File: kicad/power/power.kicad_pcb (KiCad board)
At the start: 2 copper layers, 115.3 x 75.4 mm, 31 parts, among them J1 Conn_01x06, J10 Conn_01x06, J11 Conn_01x06, J12 Conn_01x06, J13 Conn_01x06, J2 AudioJack3, J3 USB_C_Receptacle, J4 AudioJack3, J5 AudioJack3, J6 Conn_01x05_Male, J7 Screw_Terminal_01x02, J9 Conn_01x04_Male, U1 LM4565F-GE2, U2 LM4565F-GE2, U3 LM4565F-GE2, U4 LM4565F-GE2, U5 LF353DR

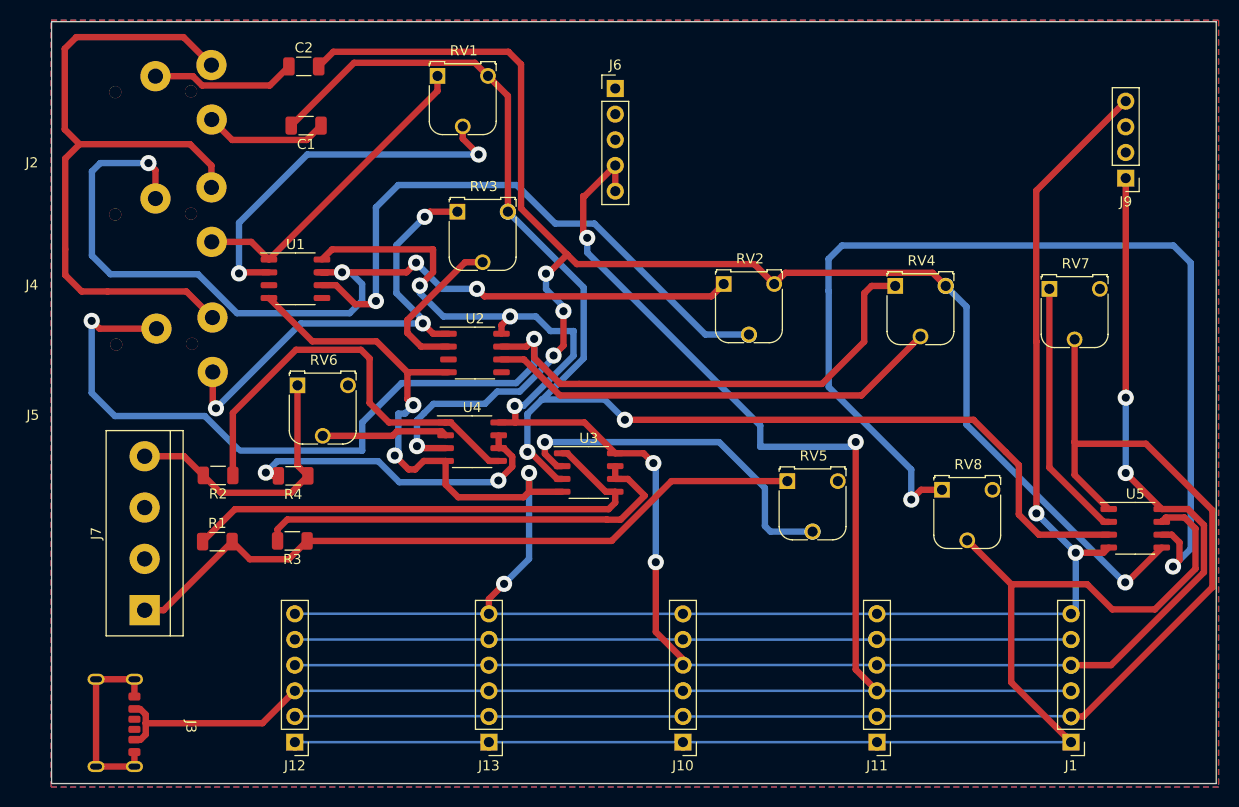
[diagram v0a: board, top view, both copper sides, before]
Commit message: Power PCB revisions
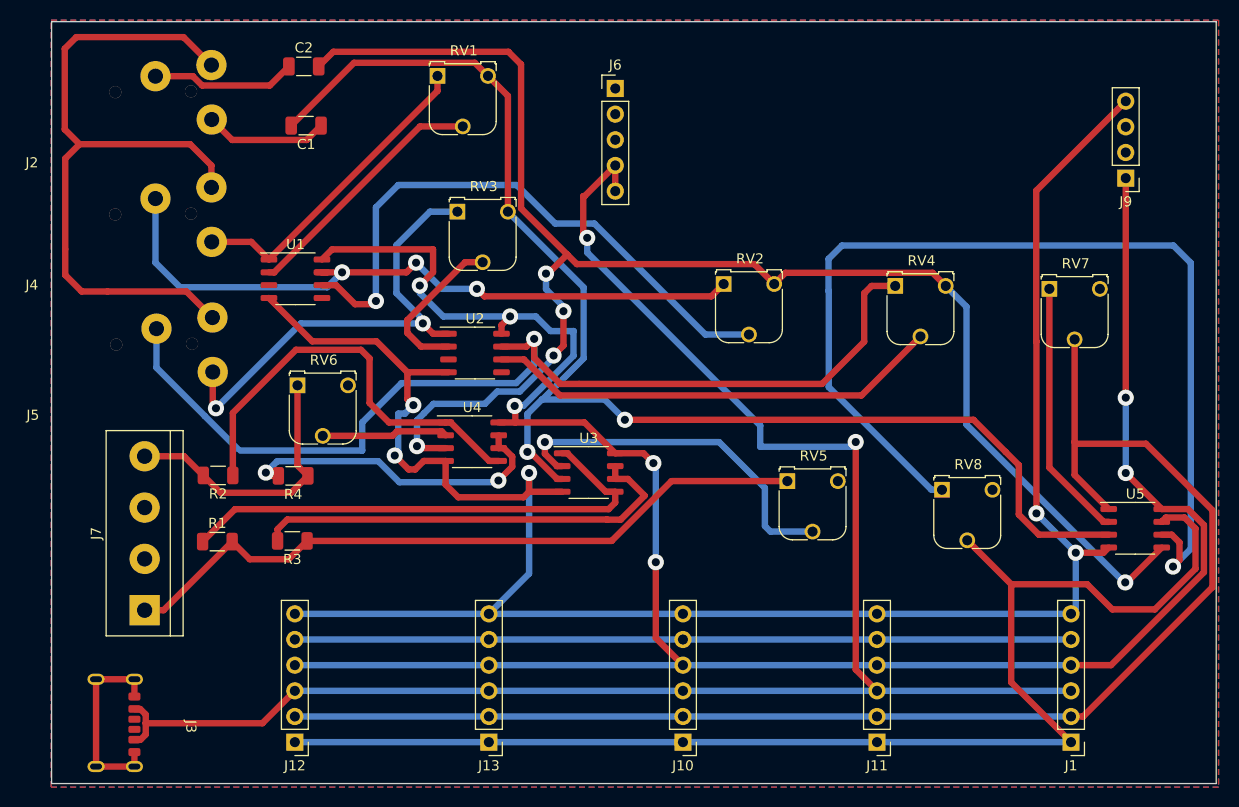
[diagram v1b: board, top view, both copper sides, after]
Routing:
- net audio_right: track 130.0 -> 206.8 mm, vias 4 -> 0
- net +5V: track 171.8 -> 248.6 mm, vias 7 -> 2
- net +15V: track 222.8 -> 299.6 mm, vias 12 -> 7
- net GND: track 168.3 -> 245.1 mm, vias 5 -> 0
- net audio_lefT: track 138.4 -> 215.0 mm, vias 5 -> 0
- net -15V: track 204.5 -> 280.6 mm, vias 11 -> 5
- net Net-(J4-PadR): track 94.9 -> 69.5 mm, vias 4 -> 3
- net Net-(J5-PadR): track 116.5 -> 101.1 mm, vias 2 -> 1
- net Net-(RV1-Pad2): track 38.0 -> 25.2 mm, vias 2 -> 0
- net Net-(RV8-Pad1): track 103.3 -> 100.7 mm, vias 2 -> 1
- net audio_in_R: vias 6 -> 5
- net audio_in_L: vias 3 -> 2
- net Net-(RV5-Pad2): vias 2 -> 1
- net Net-(RV2-Pad2): vias 2 -> 1
- net Net-(J5-PadT): vias 3 -> 2
